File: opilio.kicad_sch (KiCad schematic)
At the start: 24 parts, among them J1 Conn_01x04_Male, SW1 TS-1077S-01726, SW2 TS-1077S-01726, U1 STM32F103C8T6, Y1 YST310S 32.768KHz, Y2 TAXM8M4RFDCET2T

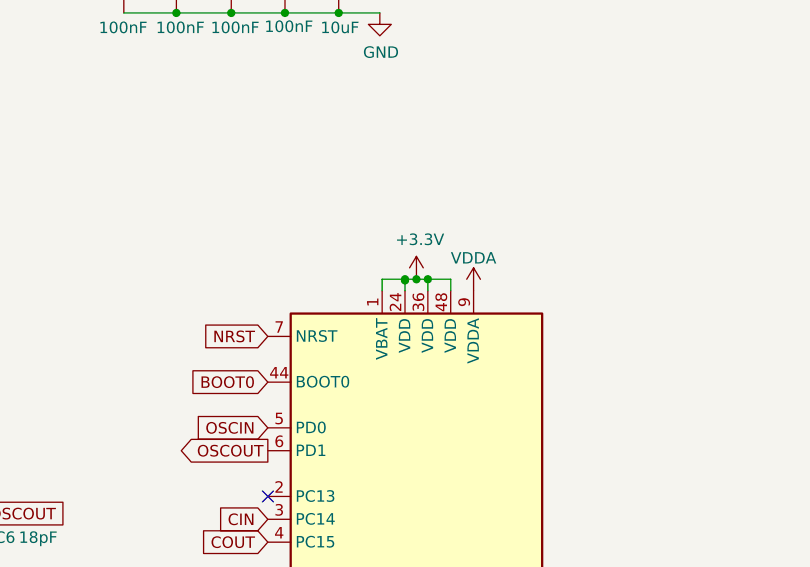
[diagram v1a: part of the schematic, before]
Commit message: kicad - 7
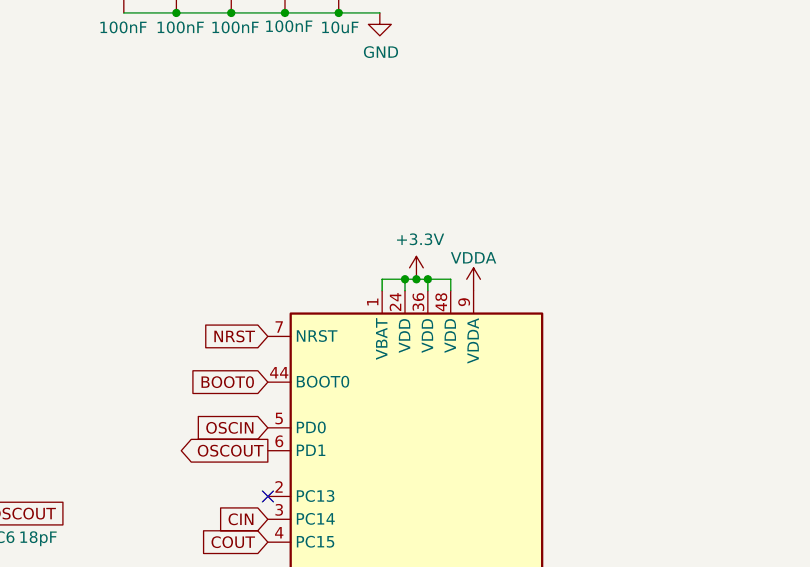
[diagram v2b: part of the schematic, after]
